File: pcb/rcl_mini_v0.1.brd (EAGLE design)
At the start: 83.8 x 64.4 mm, 60 parts, among them CN1 USB mini B, Q1 8MHz, Q2 IRLML5203, U1 MCP6002T-I/SN, U2 MCP6002T-I/SN, U3 MCP6002T-I/SN, U4 STM32F100CBT6, U5 MCP73831/OT, U6 MCP1703CB, X1 BAT, X2 TWEEZERS, X3 OLED, X4 SWD

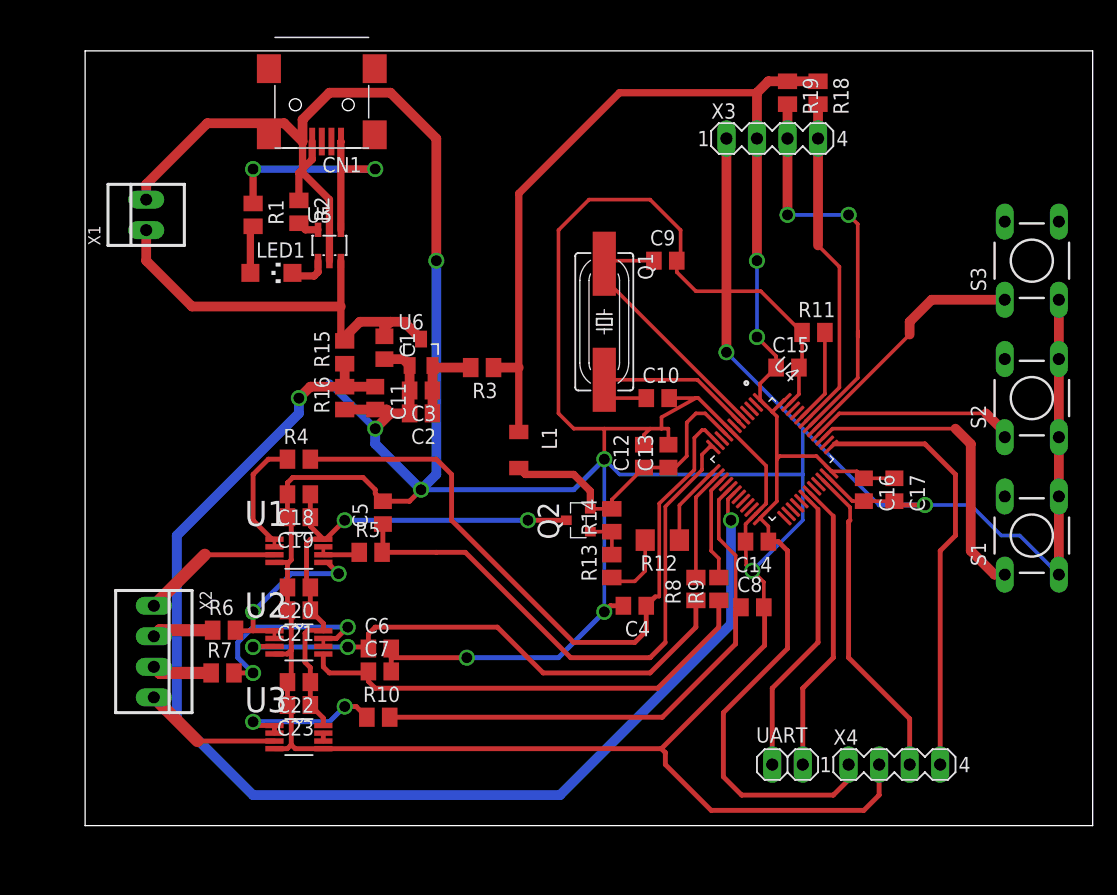
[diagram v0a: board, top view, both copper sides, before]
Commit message: pcb v1.0
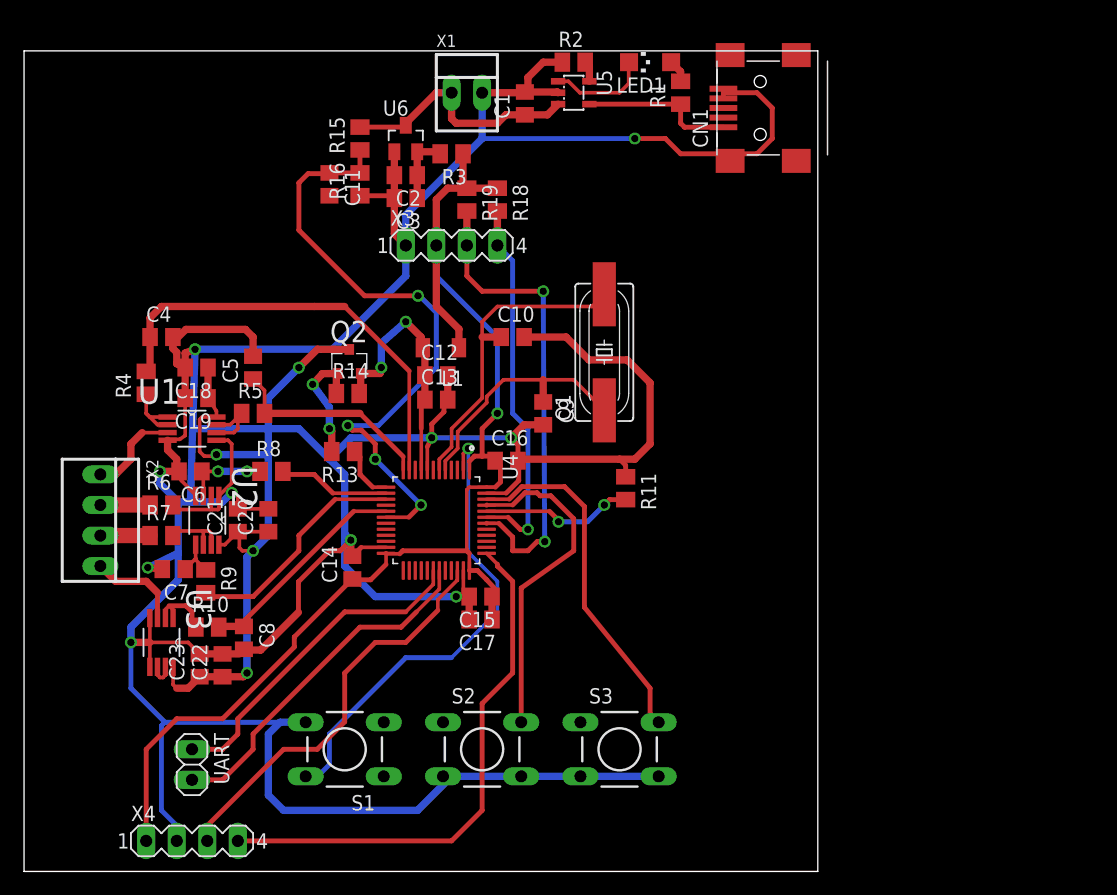
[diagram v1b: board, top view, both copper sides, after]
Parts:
- removed R12: 0, rcl:R1206
- moved S1 59.9 mm to (30.5, 41.9), turned to 180 degrees
- moved X4 58.8 mm to (17.8, 34.3)
- moved S2 54.3 mm to (41.9, 41.9), turned to 0 degrees
- moved S3 53.2 mm to (53.3, 41.9), turned to 0 degrees
- moved UART 49.5 mm to (17.8, 40.6), turned to 270 degrees
- moved C4 45.3 mm to (15.2, 76.2), turned to 0 degrees
- moved R9 42.7 mm to (18.9, 55.9), turned to 270 degrees
- moved C8 42.4 mm to (22.1, 51.2), turned to 270 degrees
- moved CN1 37.5 mm to (66.0, 95.2), turned to 90 degrees
- moved R1 37.0 mm to (58.4, 96.5), turned to 90 degrees
- moved R8 36.6 mm to (24.4, 65.0), turned to 0 degrees
- moved C17 36.1 mm to (41.8, 52.7), turned to 180 degrees
- moved LED1 36.0 mm to (55.9, 99.1), turned to 90 degrees
- moved C14 33.7 mm to (31.1, 57.0), turned to 90 degrees
- moved C15 31.9 mm to (41.8, 54.6), turned to 180 degrees
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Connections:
- removed net N$1: R12.2, R13.1
- net GND: now also S1.4, S2.4, S3.4; no longer S1.3, S2.3, S3.3
- net PA3: now also R13.1; no longer R12.1
- net SW1: now also S1.2, U4.2; no longer S1.1, U4.39
- net SW2: now also S2.2, U4.45; no longer S2.1, U4.40
- net SW3: now also S3.2, U4.46; no longer S3.1, U4.41
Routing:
- net GND: track 474.3 -> 373.7 mm, vias 9 -> 10
- net N$20: track 105.6 -> 52.6 mm, vias 2 -> 4
- net N$11: track 45.5 -> 6.91 mm
- net N$16: track 39.6 -> 3.69 mm
- net VDD: track 138.5 -> 104.5 mm, vias 2 -> 1
- net PA2: track 48.2 -> 17.4 mm
- net PA7: track 46.9 -> 18.3 mm
- net PA1: track 57.5 -> 37.0 mm
- net VCC_OPAMP: track 44.4 -> 62.0 mm, vias 2 -> 4
- net VBAT+: track 36.4 -> 21.0 mm
- net SW1: track 25.7 -> 39.7 mm, vias 0 -> 1
- net HCUR2: track 17.4 -> 5.54 mm, vias 2 -> 0
- net SW2: track 17.3 -> 27.8 mm
- net PA5: track 8.76 -> 19.2 mm
- net USB+: track 23.2 -> 12.9 mm, vias 2 -> 0
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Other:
- board size 83.8 x 64.4 mm -> 66 x 68.2 mm
